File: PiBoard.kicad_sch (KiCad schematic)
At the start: 4 parts

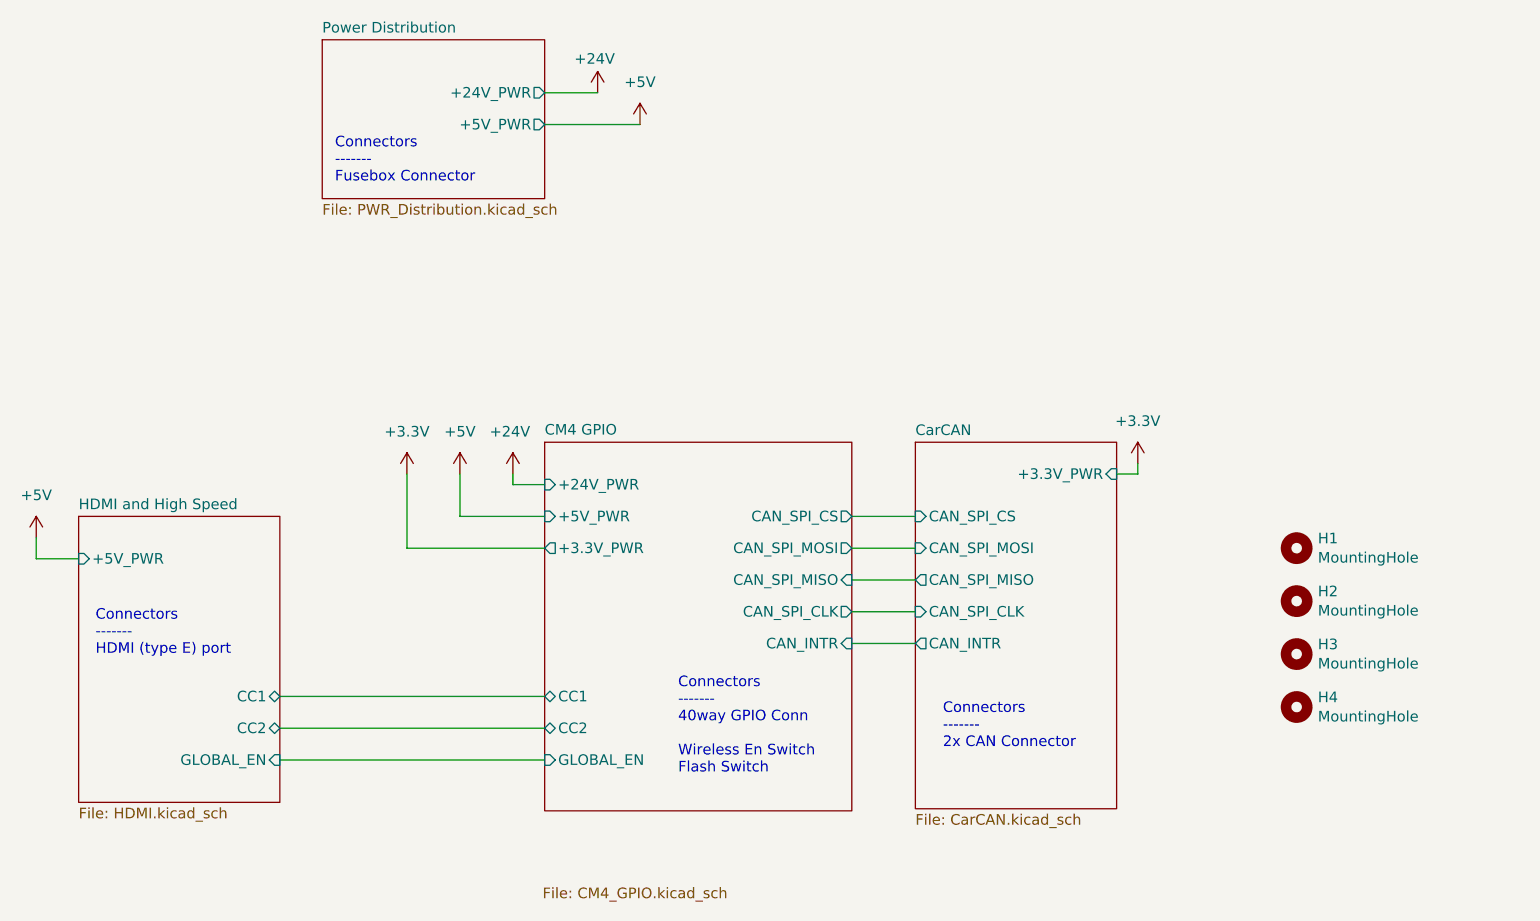
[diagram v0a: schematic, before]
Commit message: rrrrrrrr
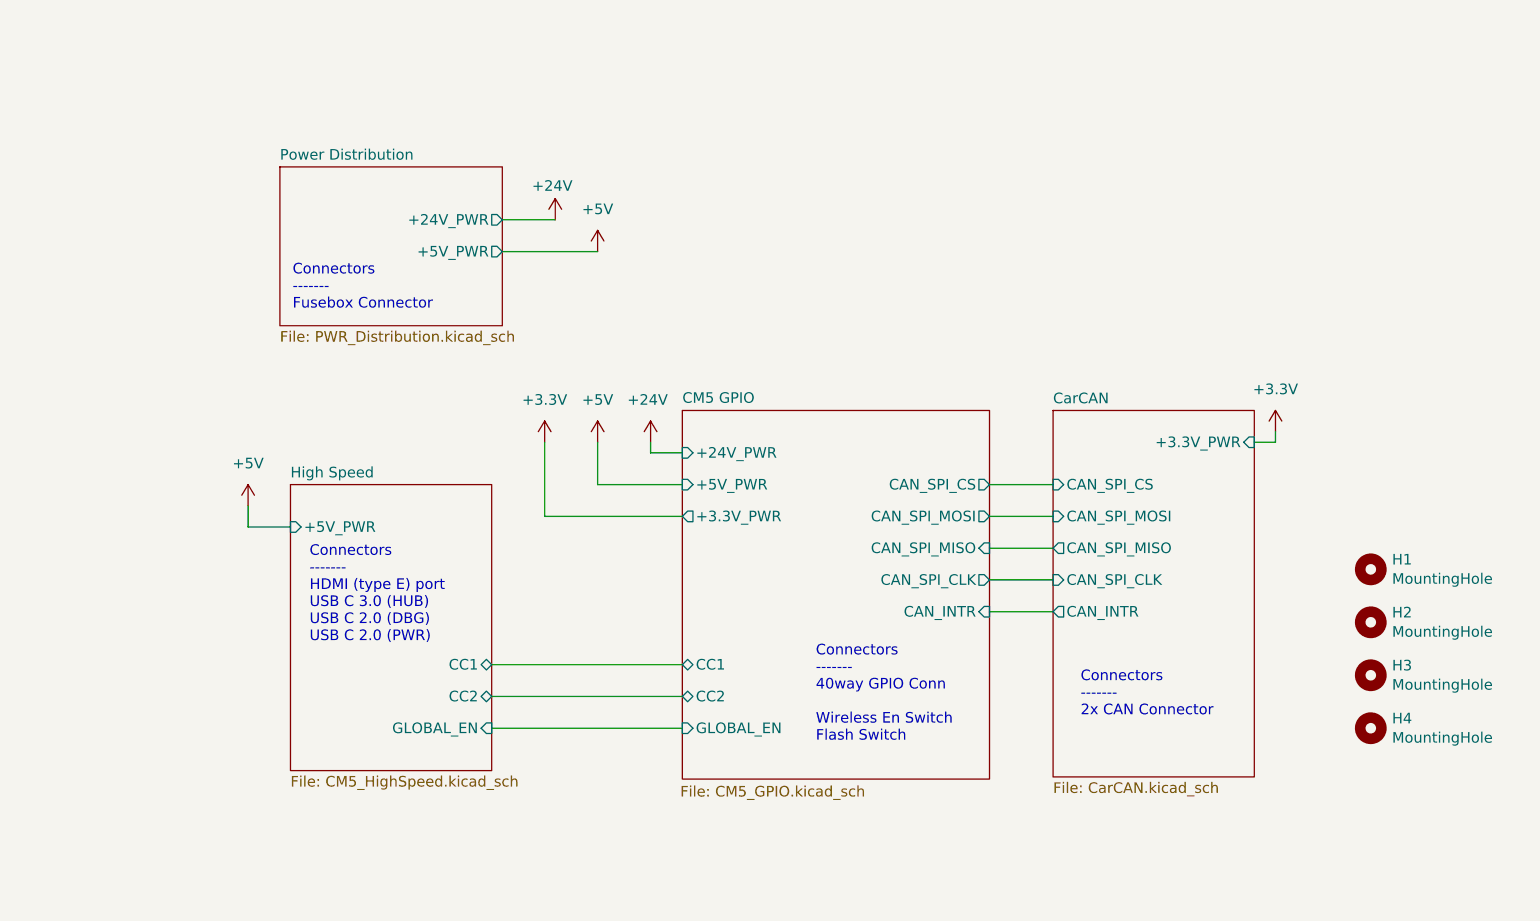
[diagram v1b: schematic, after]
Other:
- sheet CM4 GPIO renamed CM5 GPIO
- sheet HDMI and High Speed renamed High Speed
- sheet CM5 GPIO: file CM4_GPIO.kicad_sch -> CM5_GPIO.kicad_sch
- sheet High Speed: file HDMI.kicad_sch -> CM5_HighSpeed.kicad_sch
- note added: "Connectors ------- HDMI (type E) port USB C 3.0 (HUB) USB C 2.0 (DBG) USB C 2.0 (PWR)"
- note removed: "Connectors ------- HDMI (type E) port"
- moved on the sheet: H1, H2, H3, H4

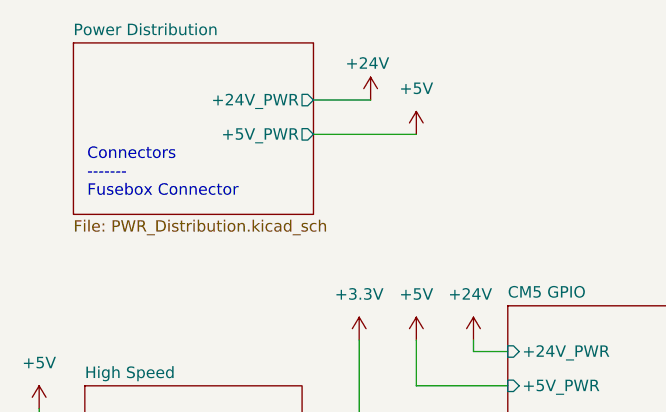
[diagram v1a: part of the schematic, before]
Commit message: Schem done? [plz full review], redoing layout
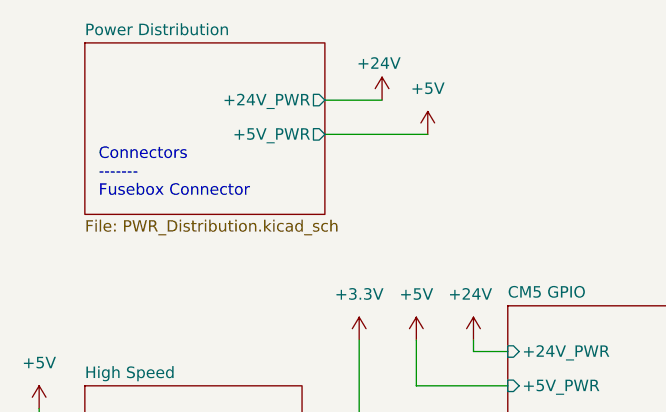
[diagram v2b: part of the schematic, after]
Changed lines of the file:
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@@
 	(text "Connectors\n-------\nFusebox Connector"
 		(exclude_from_sim no)
-		(at 86.614 71.882 0)
+		(at 87.884 71.882 0)
 		(effects
 			(font
@@
 	(wire
 		(pts
-			(xy 111.76 60.96) (xy 118.11 60.96)
+			(xy 113.03 60.96) (xy 119.38 60.96)
 		)
 		(stroke
@@
 	(wire
 		(pts
-			(xy 111.76 64.77) (xy 123.19 64.77)
+			(xy 113.03 64.77) (xy 124.46 64.77)
 		)
 		(stroke
@@
 	(symbol
 		(lib_id "power:+5V")
-		(at 123.19 64.77 0)
+		(at 124.46 64.77 0)
 		(unit 1)
 		(exclude_from_sim no)
@@
 		(fields_autoplaced yes)
 		(property "Reference" "#PWR073"
-			(at 123.19 68.58 0)
+			(at 124.46 68.58 0)
 			(effects
 				(font
@@
 		)
 		(property "Value" "+5V"
-			(at 123.19 59.69 0)
+			(at 124.46 59.69 0)
 			(effects
 				(font
@@
 		)
 		(property "Footprint" ""
-			(at 123.19 64.77 0)
+			(at 124.46 64.77 0)
 			(effects
 				(font
@@
 		)
 		(property "Datasheet" ""
-			(at 123.19 64.77 0)
+			(at 124.46 64.77 0)
 			(effects
 				(font
@@
 		)
 		(property "Description" "Power symbol creates a global label with name \"+5V\""
-			(at 123.19 64.77 0)
+			(at 124.46 64.77 0)
 			(effects
 				(font
@@
 	(symbol
 		(lib_id "power:+12V")
-		(at 118.11 60.96 0)
+		(at 119.38 60.96 0)
 		(unit 1)
 		(exclude_from_sim no)
@@
 		(dnp no)
 		(property "Reference" "#PWR066"
-			(at 118.11 64.77 0)
+			(at 119.38 64.77 0)
 			(effects
 				(font
@@
 		)
 		(property "Value" "+24V"
-			(at 115.316 56.896 0)
+			(at 116.586 56.896 0)
 			(effects
 				(font
@@
 		)
 		(property "Footprint" ""
-			(at 118.11 60.96 0)
+			(at 119.38 60.96 0)
 			(effects
 				(font
@@
 		)
 		(property "Datasheet" ""
-			(at 118.11 60.96 0)
+			(at 119.38 60.96 0)
 			(effects
 				(font
@@
 		)
 		(property "Description" "Power symbol creates a global label with name \"+12V\""
-			(at 118.11 60.96 0)
+			(at 119.38 60.96 0)
 			(effects
 				(font
@@
 	)
 	(sheet
-		(at 85.09 54.61)
+		(at 86.36 54.61)
 		(size 26.67 19.05)
 		(exclude_from_sim no)
@@
 		)
 		(property "Sheetname" "Power Distribution"
-			(at 85.09 53.8984 0)
+			(at 86.36 53.8984 0)
 			(effects
 				(font
@@
 		)
 		(property "Sheetfile" "PWR_Distribution.kicad_sch"
-			(at 85.09 74.2446 0)
+			(at 86.36 74.2446 0)
 			(effects
 				(font
@@
 		)
 		(pin "+5V_PWR" output
-			(at 111.76 64.77 0)
+			(at 113.03 64.77 0)
 			(effects
 				(font
@@
 		)
 		(pin "+24V_PWR" output
-			(at 111.76 60.96 0)
-			(effects
-				(font
+			(at 113.03 60.96 0)
+			(effects
+				(font
